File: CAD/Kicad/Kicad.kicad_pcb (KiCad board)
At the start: 2 copper layers, 25 x 40.5 mm, 33 parts, among them J1 USB_C_Receptacle_USB2.0_14P, Q1 2N3904, Q2 2N3904, SW1 SW_Push, SW2 SW_Push, U1 ESP32-S3-WROOM-2, U2 TLV75533PDRV, U9 FT231XQ

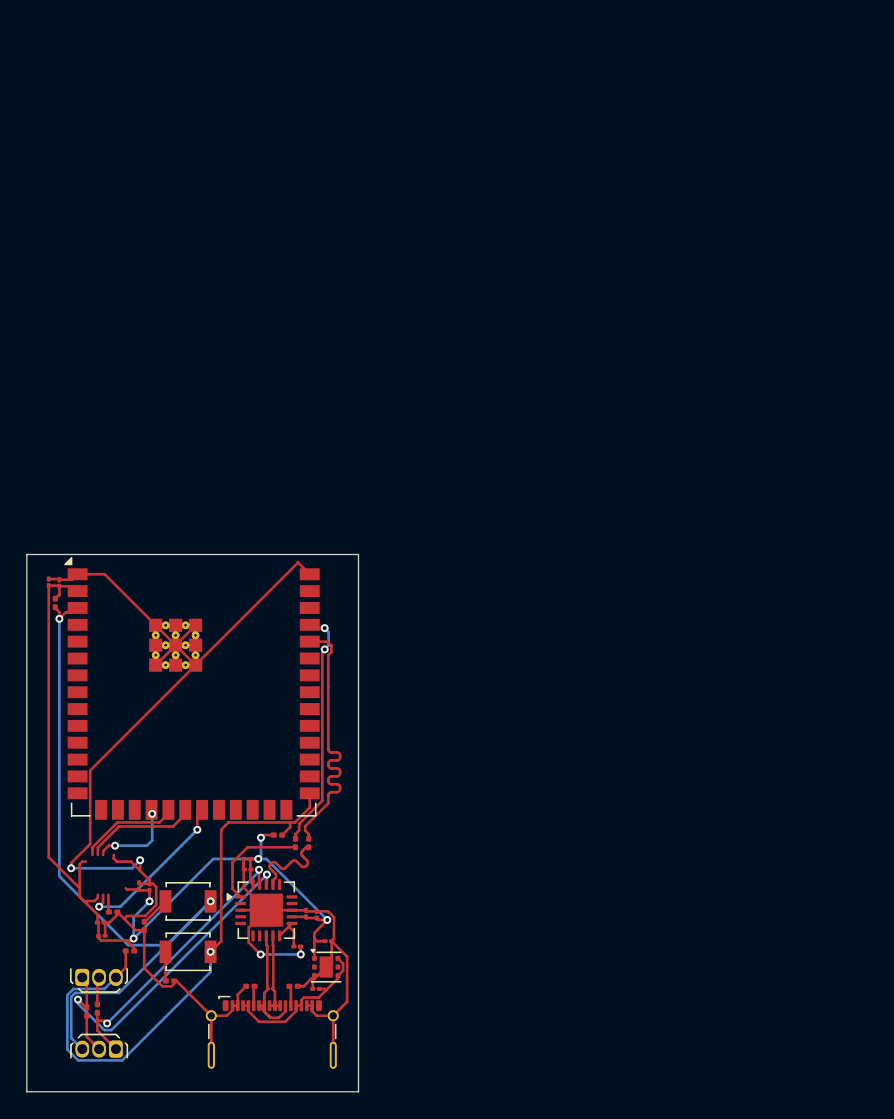
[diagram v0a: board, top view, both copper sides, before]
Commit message: finished rev4
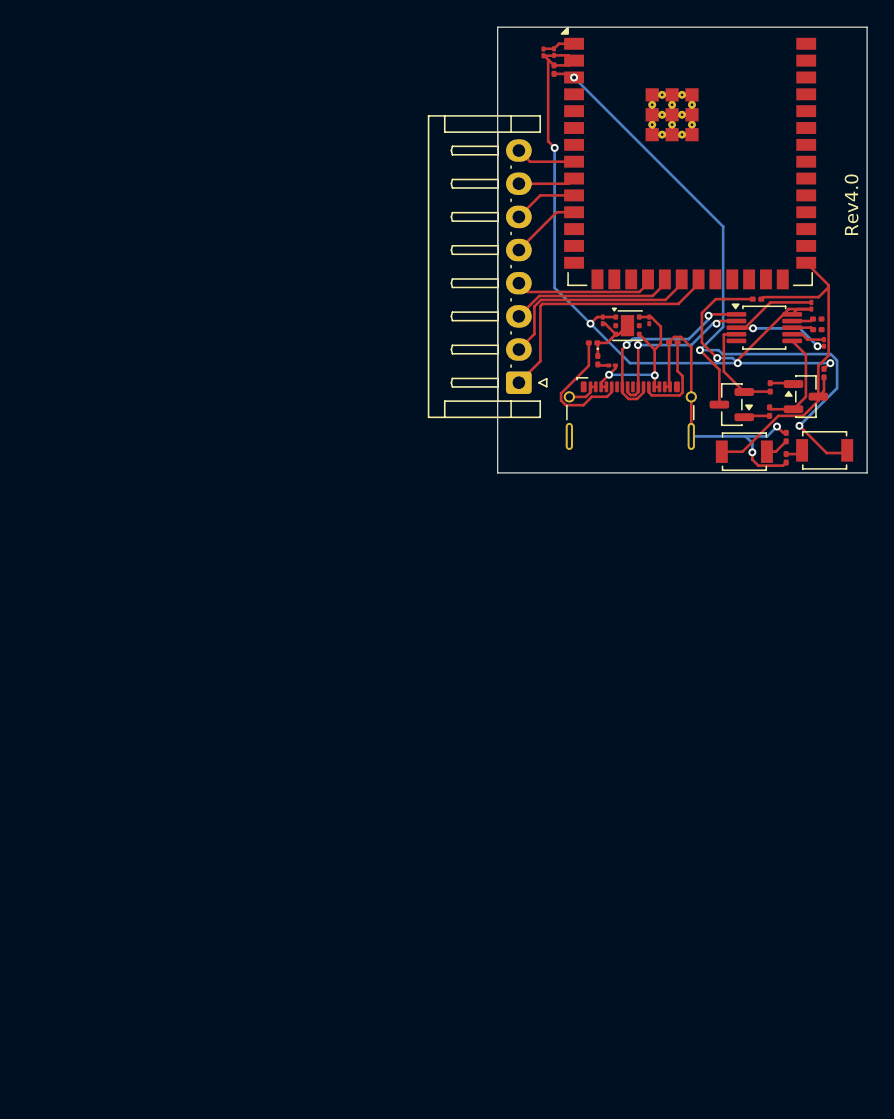
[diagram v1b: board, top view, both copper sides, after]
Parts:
- removed C10, C14, C20, C9: 0.1uF, Capacitor_SMD:C_01005_0402Metric
- removed C11: 0.1uF, Capacitor_SMD:C_0201_0603Metric
- removed C12: 22uF, Capacitor_SMD:C_01005_0402Metric
- removed C13, C15, C16, C18: 10uF, Capacitor_SMD:C_01005_0402Metric
- removed Q1, Q2: 2N3904, Package_TO_SOT_THT:TO-92Flat
- removed R16, R17: 470R, Resistor_SMD:R_0201_0603Metric
- removed U9: FT231XQ, Package_DFN_QFN:QFN-20-1EP_4x4mm_P0.5mm_EP2.5x2.5mm
- added C1: 22uF, Capacitor_SMD:C_01005_0402Metric, F.Cu at (172.0, 64.5)
- added C2: 0.1uF, Capacitor_SMD:C_01005_0402Metric, F.Cu at (172.8, 64.5)
- added D1: LED, LED_SMD:LED_0201_0603Metric, F.Cu at (176.1, 87.7)
- added J2: Conn_01x08_Socket, Connector_JST:JST_EH_S8B-EH_1x08_P2.50mm_Horizontal, F.Cu at (170.2, 89.4)
- added Q3: MMBT3904, Package_TO_SOT_SMD:SOT-23, F.Cu at (186.2, 91.0)
- added Q4: MMBT3904, Package_TO_SOT_SMD:SOT-23, F.Cu at (191.8, 90.5)
- added R10: 5K1, Resistor_SMD:R_0201_0603Metric, F.Cu at (175.7, 86.4)
- added R11: 5K1, Resistor_SMD:R_0201_0603Metric, F.Cu at (181.8, 86.3)
- added R12: 150R, Resistor_SMD:R_01005_0402Metric, F.Cu at (177.2, 88.1)
- added U3: CH340X, Package_SO:MSOP-10_3x3mm_P0.5mm, F.Cu at (188.7, 85.2)
- R1, R2: value 5K1 -> 12K
- R3: value 10K -> 4K1
- R5, R6: value 12K -> 10K
- R7: value 4.7K -> 12K
- R8: value 12K -> 470R
- R9: value 10K -> 470R
- moved R5 79.3 mm to (172.8, 65.8)
- moved R6 73.0 mm to (188.1, 83.1), turned to 0 degrees
- moved R8 69.8 mm to (192.6, 84.6)
- moved R7 62.8 mm to (190.3, 93.5), turned to -90 degrees
- moved R3 60.5 mm to (193.2, 88.7), turned to 90 degrees
- moved C3 60.4 mm to (192.2, 83.6)
- moved C4 60.4 mm to (193.2, 86.4), turned to 90 degrees
- moved R4 59.9 mm to (190.3, 95.1), turned to 90 degrees
- moved SW1 58.8 mm to (193.2, 94.5)
- moved R1 58.4 mm to (189.1, 91.6), turned to -90 degrees
- moved R2 57.7 mm to (189.1, 89.8), turned to 90 degrees
- moved SW2 56.4 mm to (187.2, 94.6), turned to 0 degrees
- moved R9 55.7 mm to (192.7, 85.4), turned to 180 degrees
- moved C5 54.8 mm to (176.5, 84.7), turned to -90 degrees
- moved U1 54.8 mm to (183.1, 69.1)
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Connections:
- C3 pad 2: /VCC0 -> VCC
- C4 pad 1: /VCC0 -> GND
- C4 pad 2: GND -> Net-(U3-VCC)
- C5 pad 1: /5V_USB_1 -> VCC
- C6 pad 1: /VCC0 -> /5V_USB_1
- R1 pad 1: Net-(J1-CC1) -> /DTR
- R1 pad 2: GND -> Net-(Q3-B)
- R2 pad 1: Net-(J1-CC2) -> /RTS
- R2 pad 2: GND -> Net-(Q4-B)
- R3 pad 1: /VCC0 -> /BOOT
- R3 pad 2: /ESP32_AUTORST -> VCC
- R4 pad 1: Net-(R4-Pad1) -> GND
- R4 pad 2: GND -> Net-(R4-Pad2)
- R5 pad 1: /DTR_A -> VCC
- R5 pad 2: Net-(Q2-B) -> /ESP32_AUTORST
- R6 pad 1: /RTS_A -> VCC
- R6 pad 2: Net-(Q1-B) -> /BOOT
- R7 pad 1: /BOOT -> GND
- R7 pad 2: /VCC0 -> Net-(R7-Pad2)
- R8 pad 1: GND -> Net-(U1-TXD0/IO43)
- R8 pad 2: Net-(R8-Pad2) -> /ESP32_SERIAL_P
- R9 pad 1: /VCC0 -> Net-(U1-RXD0/IO44)
- R9 pad 2: /BOOT -> /ESP32_SERIAL_N
- SW1 pad 1: Net-(R4-Pad1) -> Net-(R4-Pad2)
- SW2 pad 2: Net-(R8-Pad2) -> Net-(R7-Pad2)
- U1 pad 12: /IO8 -> unconnected-(U1-IO8-Pad12)
- U1 pad 15: /IO3 -> unconnected-(U1-IO3-Pad15)
- U1 pad 16: /IO46 -> unconnected-(U1-IO46-Pad16)
- U1 pad 17: /IO9 -> unconnected-(U1-IO9-Pad17)
- U1 pad 18: /CS_BUS_A -> /CS
- U1 pad 19: /MOSI_BUS_A -> /MOSI
- U1 pad 2: /VCC0 -> VCC
- U1 pad 20: /SCK_BUS_A -> /SCK
- U1 pad 21: /MISO_BUS_A -> /MISO
- U1 pad 22: /IO14 -> unconnected-(U1-IO14-Pad22)
- U1 pad 23: /IO21 -> unconnected-(U1-IO21-Pad23)
- U1 pad 24: /IO47 -> unconnected-(U1-IO47-Pad24)
- U1 pad 25: /IO48 -> unconnected-(U1-IO48-Pad25)
- U1 pad 26: /IO45 -> unconnected-(U1-IO45-Pad26)
- U1 pad 31: /IO38 -> unconnected-(U1-IO38-Pad31)
- U1 pad 32: /IO39 -> unconnected-(U1-MTCK/IO39-Pad32)
- U1 pad 33: /IO40 -> unconnected-(U1-MTDO/IO40-Pad33)
- U1 pad 34: /IO41 -> unconnected-(U1-MTDI/IO41-Pad34)
- U1 pad 35: /IO42 -> unconnected-(U1-MTMS/IO42-Pad35)
- U1 pad 38: /IO2 -> unconnected-(U1-IO2-Pad38)
- U1 pad 39: /IO1 -> unconnected-(U1-IO1-Pad39)
- U1 pad 4: /IO4 -> unconnected-(U1-IO4-Pad4)
- U1 pad 5: /IO5 -> unconnected-(U1-IO5-Pad5)
- U1 pad 6: /IO6 -> unconnected-(U1-IO6-Pad6)
- U1 pad 7: /IO7 -> unconnected-(U1-IO7-Pad7)
- U2 pad 1: /VCC0 -> VCC
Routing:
- net GND: track 135.0 -> 48.9 mm
- net /VCC0: track 79.8 -> 0.00 mm, vias 5 -> 0
- net VCC: track 0.00 -> 67.4 mm, vias 0 -> 5
- net /DTR_A: track 24.4 -> 0.00 mm, vias 2 -> 0
- net /RTS_A: track 21.6 -> 0.00 mm, vias 2 -> 0
- net Net-(U1-RXD0/IO44): track 21.2 -> 0.00 mm
- net /MISO: track 0.00 -> 19.4 mm
- net Net-(U1-TXD0/IO43): track 18.3 -> 0.00 mm, vias 2 -> 0
- net /BOOT: track 45.2 -> 27.4 mm, vias 1 -> 0
- net /SCK: track 0.00 -> 15.9 mm
- net /MISO_BUS_A: track 12.5 -> 0.00 mm, vias 2 -> 0
- net /MOSI: track 0.00 -> 12.4 mm
- net /CS: track 0.00 -> 10.6 mm
- net Net-(J1-CC1): track 1.49 -> 10.1 mm
- net /SCK_BUS_A: track 8.51 -> 0.00 mm
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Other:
- board size 25 x 40.5 mm -> 27.8 x 33.6 mm
- board text added: "Rev4.0"
- board text removed: "Designed By Matias Argandona Rev3.1"

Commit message: fixed BOM and markdown typo
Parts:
- R12: value 150R -> 200R
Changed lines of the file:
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@@
 			)
 		)
-		(property "LCSC Part #" "C4109"
+		(property "LCSC Part #" "C131361"
 			(at 0 0 0)
 			(unlocked yes)
@@
 			)
 		)
-		(property "Value" "150R"
+		(property "Value" "200R"
 			(at 0 1 0)
 			(layer "F.Fab")
@@
 			)
 		)
-		(property "LCSC Part #" "C4109"
+		(property "LCSC Part #" "C25087"
 			(at 0 0 180)
 			(unlocked yes)
@@
 			)
 		)
-		(property "LCSC Part #" "C4109"
+		(property "LCSC Part #" "C131361"
 			(at 0 0 270)
 			(unlocked yes)
